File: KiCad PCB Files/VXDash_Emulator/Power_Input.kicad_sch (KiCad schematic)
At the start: 18 parts, among them Q10 2N7002, Q11 PJA3441, Q12 PJA3441

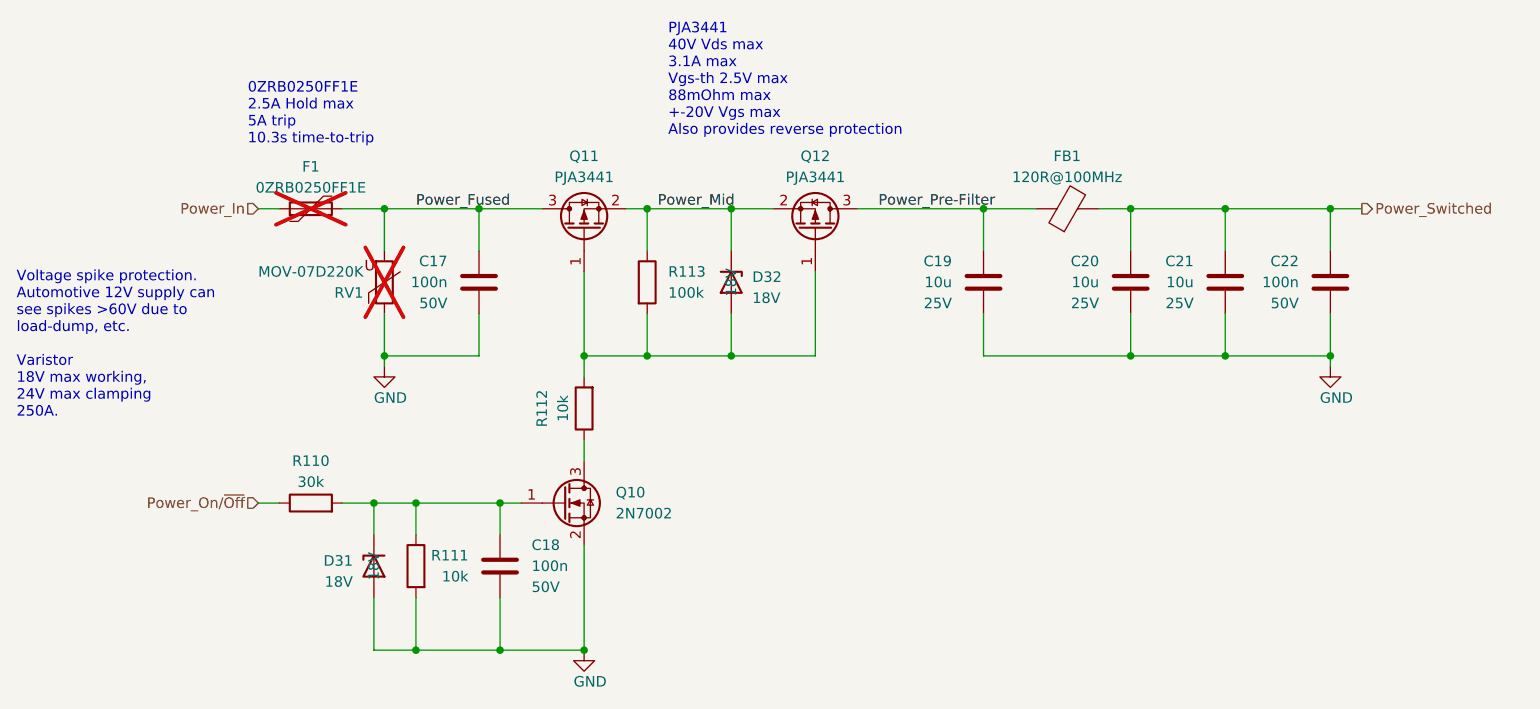
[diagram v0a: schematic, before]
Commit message: Emulator : LCSC part numbers and production files
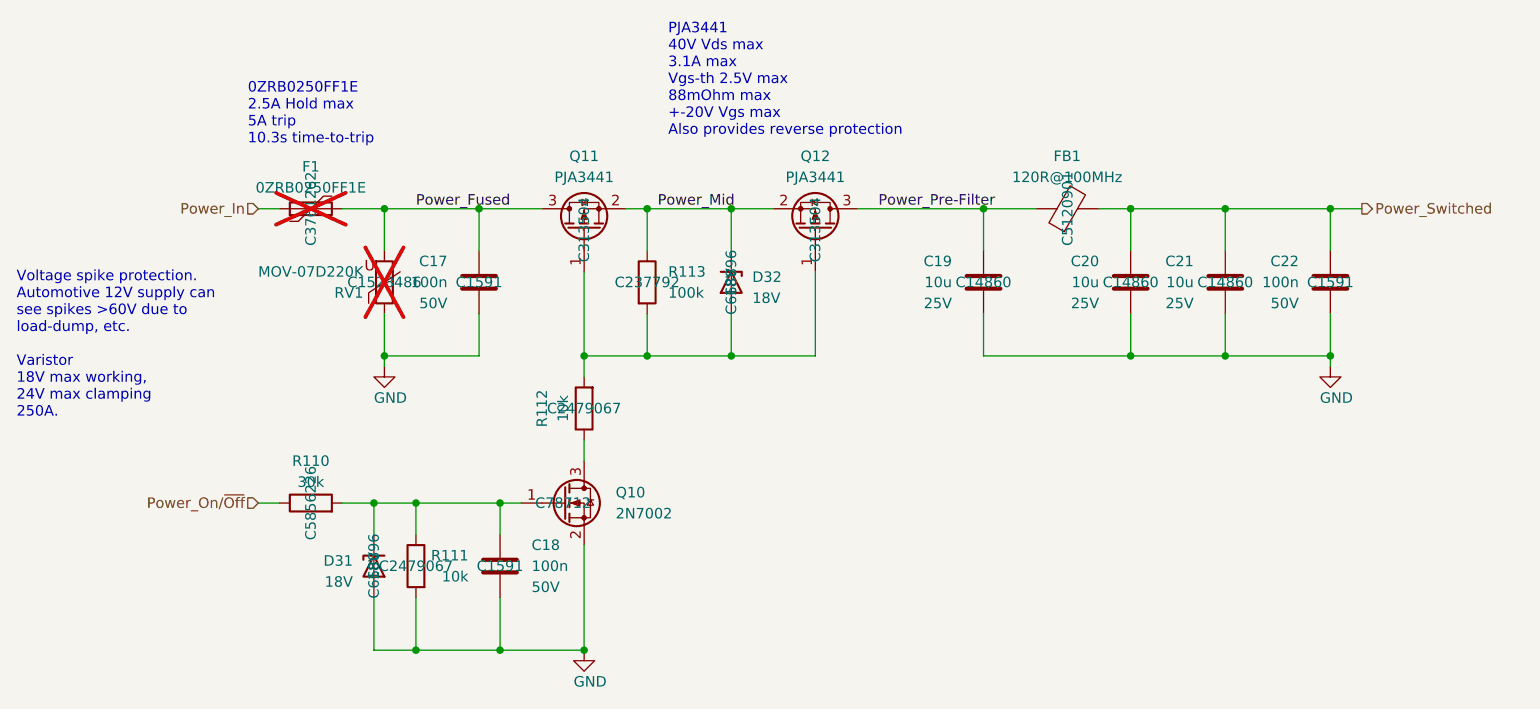
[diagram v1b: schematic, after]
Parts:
- C17, C18, C22: LCSC (none) -> C1591; MFT_PN CL10B104KB8NNWC -> CL10B104KB8NNNC
- C19, C20, C21: LCSC (none) -> C14860
- D31, D32: LCSC (none) -> C668896
- F1: LCSC (none) -> C3761262
- FB1: LCSC (none) -> C5120901
- Q10: LCSC (none) -> C78712
- Q11, Q12: LCSC (none) -> C313504
- R110: LCSC (none) -> C5856226
- R111, R112: LCSC (none) -> C2479067
- R113: LCSC (none) -> C237792
- RV1: LCSC (none) -> C1528486
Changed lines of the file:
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@@
+			)
+		)
+		(property "LCSC" "C2479067"
+			(at 132.08 99.06 0)
+			(effects
+				(font
+					(size 1.27 1.27)
+				)
 			)
 		)
@@
 			)
 		)
-		(property "MFT_PN" "CL10B104KB8NNWC"
+		(property "MFT_PN" "CL10B104KB8NNNC"
 			(at 222.25 83.82 0)
 			(effects
@@
 				)
 				(hide yes)
+			)
+		)
+		(property "LCSC" "C1591"
+			(at 222.25 83.82 0)
+			(effects
+				(font
+					(size 1.27 1.27)
+				)
 			)
 		)
@@
 			)
 		)
+		(property "LCSC" "C5120901"
+			(at 190.5 74.93 0)
+			(effects
+				(font
+					(size 1.27 1.27)
+				)
+			)
+		)
 		(pin "1"
 		)
@@
 				)
 				(hide yes)
+			)
+		)
+		(property "LCSC" "C313504"
+			(at 132.08 77.47 0)
+			(effects
+				(font
+					(size 1.27 1.27)
+				)
 			)
 		)
@@
 			)
 		)
-		(property "MFT_PN" "CL10B104KB8NNWC"
+		(property "MFT_PN" "CL10B104KB8NNNC"
 			(at 119.38 83.82 0)
 			(effects
@@
 				)
 				(hide yes)
+			)
+		)
+		(property "LCSC" "C1591"
+			(at 119.38 83.82 0)
+			(effects
+				(font
+					(size 1.27 1.27)
+				)
 			)
 		)
@@
 			)
 		)
+		(property "LCSC" "C2479067"
+			(at 111.76 118.11 0)
+			(effects
+				(font
+					(size 1.27 1.27)
+				)
+			)
+		)
 		(pin "1"
 		)
@@
 			)
 		)
+		(property "LCSC" "C668896"
+			(at 149.86 83.82 0)
+			(effects
+				(font
+					(size 1.27 1.27)
+				)
+			)
+		)
 		(pin "1"
 		)
@@
 				)
 				(hide yes)
+			)
+		)
+		(property "LCSC" "C5856226"
+			(at 99.06 110.49 0)
+			(effects
+				(font
+					(size 1.27 1.27)
+				)
 			)
 		)
@@
 			)
 		)
+		(property "LCSC" "C313504"
+			(at 160.02 77.47 0)
+			(effects
+				(font
+					(size 1.27 1.27)
+				)
+			)
+		)
 		(pin "1"
 		)
@@
 				)
 				(hide yes)
+			)
+		)
+		(property "LCSC" "C78712"
+			(at 129.54 110.49 0)
+			(effects
+				(font
+					(size 1.27 1.27)
+				)
 			)
 		)
@@
 			)
 		)
+		(property "LCSC" "C14860"
+			(at 198.12 83.82 0)
+			(effects
+				(font
+					(size 1.27 1.27)
+				)
+			)
+		)
 		(pin "1"
 		)
@@
 			)
 		)
-		(property "MFT_PN" "CL10B104KB8NNWC"
+		(property "MFT_PN" "CL10B104KB8NNNC"
 			(at 121.92 118.11 0)
 			(effects
@@
 				)
 				(hide yes)
+			)
+		)
+		(property "LCSC" "C1591"
+			(at 121.92 118.11 0)
+			(effects
+				(font
+					(size 1.27 1.27)
+				)
 			)
 		)
@@
 			)
 		)
+		(property "LCSC" "C668896"
+			(at 106.68 118.11 0)
+			(effects
+				(font
+					(size 1.27 1.27)
+				)
+			)
+		)
 		(pin "1"
 		)
@@
 			)
 		)
+		(property "LCSC" "C237792"
+			(at 139.7 83.82 0)
+			(effects
+				(font
+					(size 1.27 1.27)
+				)
+			)
+		)
 		(pin "1"
 		)
@@
 				)
 				(hide yes)
+			)
+		)
+		(property "LCSC" "C3761262"
+			(at 99.06 74.93 0)
+			(effects
+				(font
+					(size 1.27 1.27)
+				)
 			)
 		)
@@
 			)
 		)
+		(property "LCSC" "C14860"
+			(at 180.34 83.82 0)
+			(effects
+				(font
+					(size 1.27 1.27)
+				)
+			)
+		)
 		(pin "1"
 		)
@@
 			)
 		)
+		(property "LCSC" "C14860"
+			(at 209.55 83.82 0)
+			(effects
+				(font
+					(size 1.27 1.27)
+				)
+			)
+		)
 		(pin "1"
 		)
@@
 			)
 		)
+		(property "LCSC" "C1528486"
+			(at 107.95 83.82 0)
+			(effects
+				(font
+					(size 1.27 1.27)
+				)
+			)
+		)

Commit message: Emulator : Updating BOM with LCSC alts
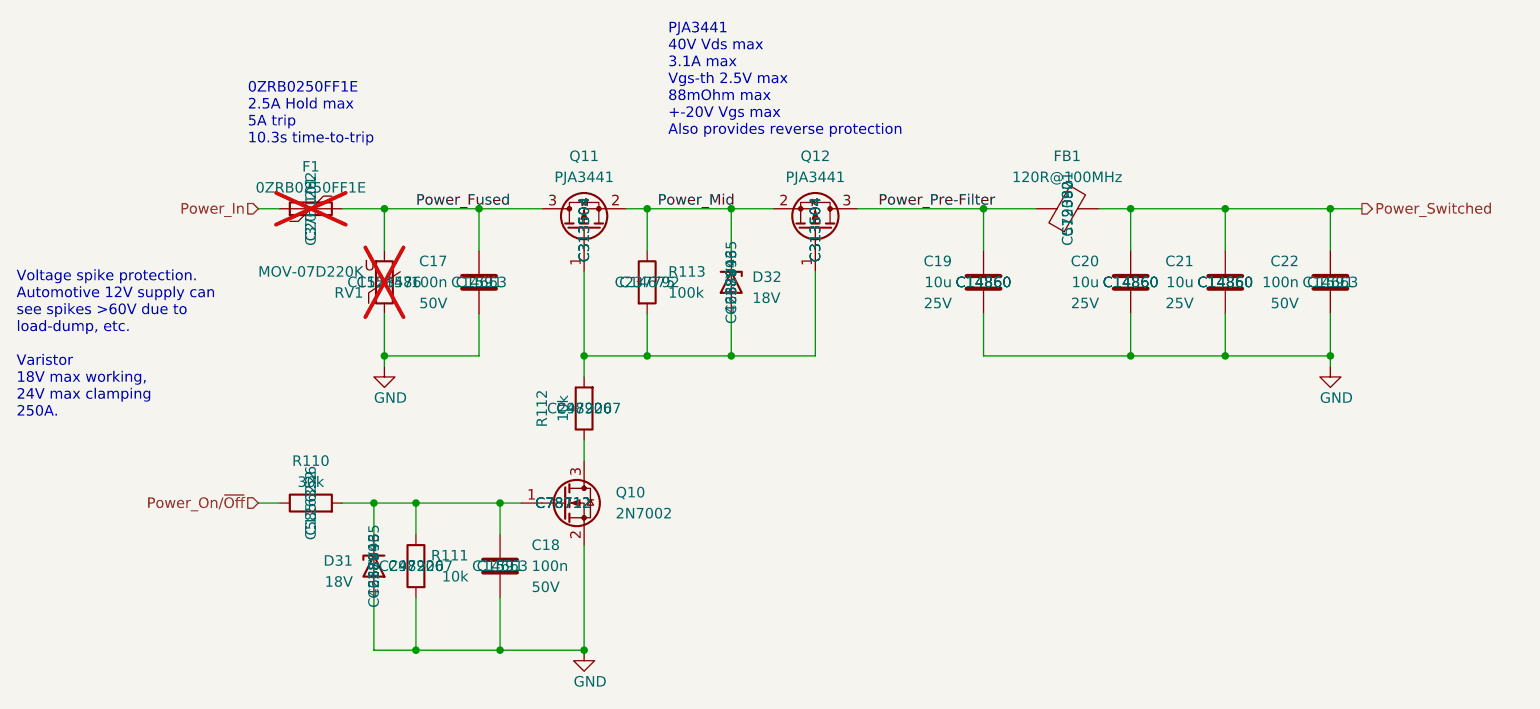
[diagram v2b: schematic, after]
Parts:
- C17, C18, C22: LCSC alt (none) -> C14663
- C19, C20, C21: LCSC alt (none) -> C14860
- D31, D32: LCSC alt (none) -> C42379435
- F1: LCSC alt (none) -> C207101
- FB1: LCSC alt (none) -> C79382
- Q10: LCSC alt (none) -> C78712
- Q11, Q12: LCSC alt (none) -> C313504
- R110: LCSC alt (none) -> C126352
- R111, R112: LCSC alt (none) -> C98220
- R113: LCSC alt (none) -> C14675
- RV1: LCSC alt (none) -> C15157
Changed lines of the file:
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@@
+			)
+		)
+		(property "LCSC alt" "C98220"
+			(at 132.08 99.06 0)
+			(effects
+				(font
+					(size 1.27 1.27)
+				)
 			)
 		)
@@
 			)
 		)
+		(property "LCSC alt" "C14663"
+			(at 222.25 83.82 0)
+			(effects
+				(font
+					(size 1.27 1.27)
+				)
+			)
+		)
 		(pin "1"
 		)
@@
 			)
 		)
+		(property "LCSC alt" "C79382"
+			(at 190.5 74.93 0)
+			(effects
+				(font
+					(size 1.27 1.27)
+				)
+			)
+		)
 		(pin "1"
 		)
@@
 		)
 		(property "LCSC" "C313504"
+			(at 132.08 77.47 0)
+			(effects
+				(font
+					(size 1.27 1.27)
+				)
+			)
+		)
+		(property "LCSC alt" "C313504"
 			(at 132.08 77.47 0)
 			(effects
@@
 			)
 		)
+		(property "LCSC alt" "C14663"
+			(at 119.38 83.82 0)
+			(effects
+				(font
+					(size 1.27 1.27)
+				)
+			)
+		)
 		(pin "1"
 		)
@@
 			)
 		)
+		(property "LCSC alt" "C98220"
+			(at 111.76 118.11 0)
+			(effects
+				(font
+					(size 1.27 1.27)
+				)
+			)
+		)
 		(pin "1"
 		)
@@
 			)
 		)
+		(property "LCSC alt" "C42379435"
+			(at 149.86 83.82 0)
+			(effects
+				(font
+					(size 1.27 1.27)
+				)
+			)
+		)
 		(pin "1"
 		)
@@
 		)
 		(property "LCSC" "C5856226"
+			(at 99.06 110.49 0)
+			(effects
+				(font
+					(size 1.27 1.27)
+				)
+			)
+		)
+		(property "LCSC alt" "C126352"
 			(at 99.06 110.49 0)
 			(effects
@@
 			)
 		)
+		(property "LCSC alt" "C313504"
+			(at 160.02 77.47 0)
+			(effects
+				(font
+					(size 1.27 1.27)
+				)
+			)
+		)
 		(pin "1"
 		)
@@
 		)
 		(property "LCSC" "C78712"
+			(at 129.54 110.49 0)
+			(effects
+				(font
+					(size 1.27 1.27)
+				)
+			)
+		)
+		(property "LCSC alt" "C78712"
 			(at 129.54 110.49 0)
 			(effects
@@
 			)
 		)
+		(property "LCSC alt" "C14860"
+			(at 198.12 83.82 0)
+			(effects
+				(font
+					(size 1.27 1.27)
+				)
+			)
+		)
 		(pin "1"
 		)
@@
 		)
 		(property "LCSC" "C1591"
+			(at 121.92 118.11 0)
+			(effects
+				(font
+					(size 1.27 1.27)
+				)
+			)
+		)
+		(property "LCSC alt" "C14663"
 			(at 121.92 118.11 0)
 			(effects
@@
 			)
 		)
+		(property "LCSC alt" "C42379435"
+			(at 106.68 118.11 0)
+			(effects
+				(font
+					(size 1.27 1.27)
+				)
+			)
+		)
 		(pin "1"
 		)
@@
 			)
 		)
+		(property "LCSC alt" "C14675"
+			(at 139.7 83.82 0)
+			(effects
+				(font
+					(size 1.27 1.27)
+				)
+			)
+		)
 		(pin "1"
 		)
@@
 		)
 		(property "LCSC" "C3761262"
+			(at 99.06 74.93 0)
+			(effects
+				(font
+					(size 1.27 1.27)
+				)
+			)
+		)
+		(property "LCSC alt" "C207101"
 			(at 99.06 74.93 0)
 			(effects
@@
 			)
 		)
+		(property "LCSC alt" "C14860"
+			(at 180.34 83.82 0)
+			(effects
+				(font
+					(size 1.27 1.27)
+				)
+			)
+		)
 		(pin "1"
 		)
@@
 			)
 		)
+		(property "LCSC alt" "C14860"
+			(at 209.55 83.82 0)
+			(effects
+				(font
+					(size 1.27 1.27)
+				)
+			)
+		)
 		(pin "1"
 		)
@@
 			(at 107.95 83.82 0)
 			(effects
+				(font
+					(size 1.27 1.27)
+				)
+			)
+		)
+		(property "LCSC alt" "C15157"
+			(at 107.95 83.82 0)
+			(effects
